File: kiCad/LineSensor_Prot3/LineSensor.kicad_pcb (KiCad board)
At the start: 2 copper layers, 113 parts, among them J1 Conn_01x04_Socket, J2 Conn_01x02_Socket, Q1 Q_Photo_NPN, Q10 Q_Photo_NPN, Q11 Q_Photo_NPN, Q12 Q_Photo_NPN, Q13 Q_Photo_NPN, Q14 Q_Photo_NPN, Q15 Q_Photo_NPN, Q16 Q_Photo_NPN, Q17 NMOS, Q2 Q_Photo_NPN, Q3 Q_Photo_NPN, Q4 Q_Photo_NPN, Q5 Q_Photo_NPN, Q6 Q_Photo_NPN, Q7 Q_Photo_NPN, Q8 Q_Photo_NPN, Q9 Q_Photo_NPN, SW2 SW_DPST_x2, U1 LM393, U2 LM393, U3 LM393, U4 LM393, U5 LM393, U6 LM393, U7 LM393, U8 LM393, U9 LM393

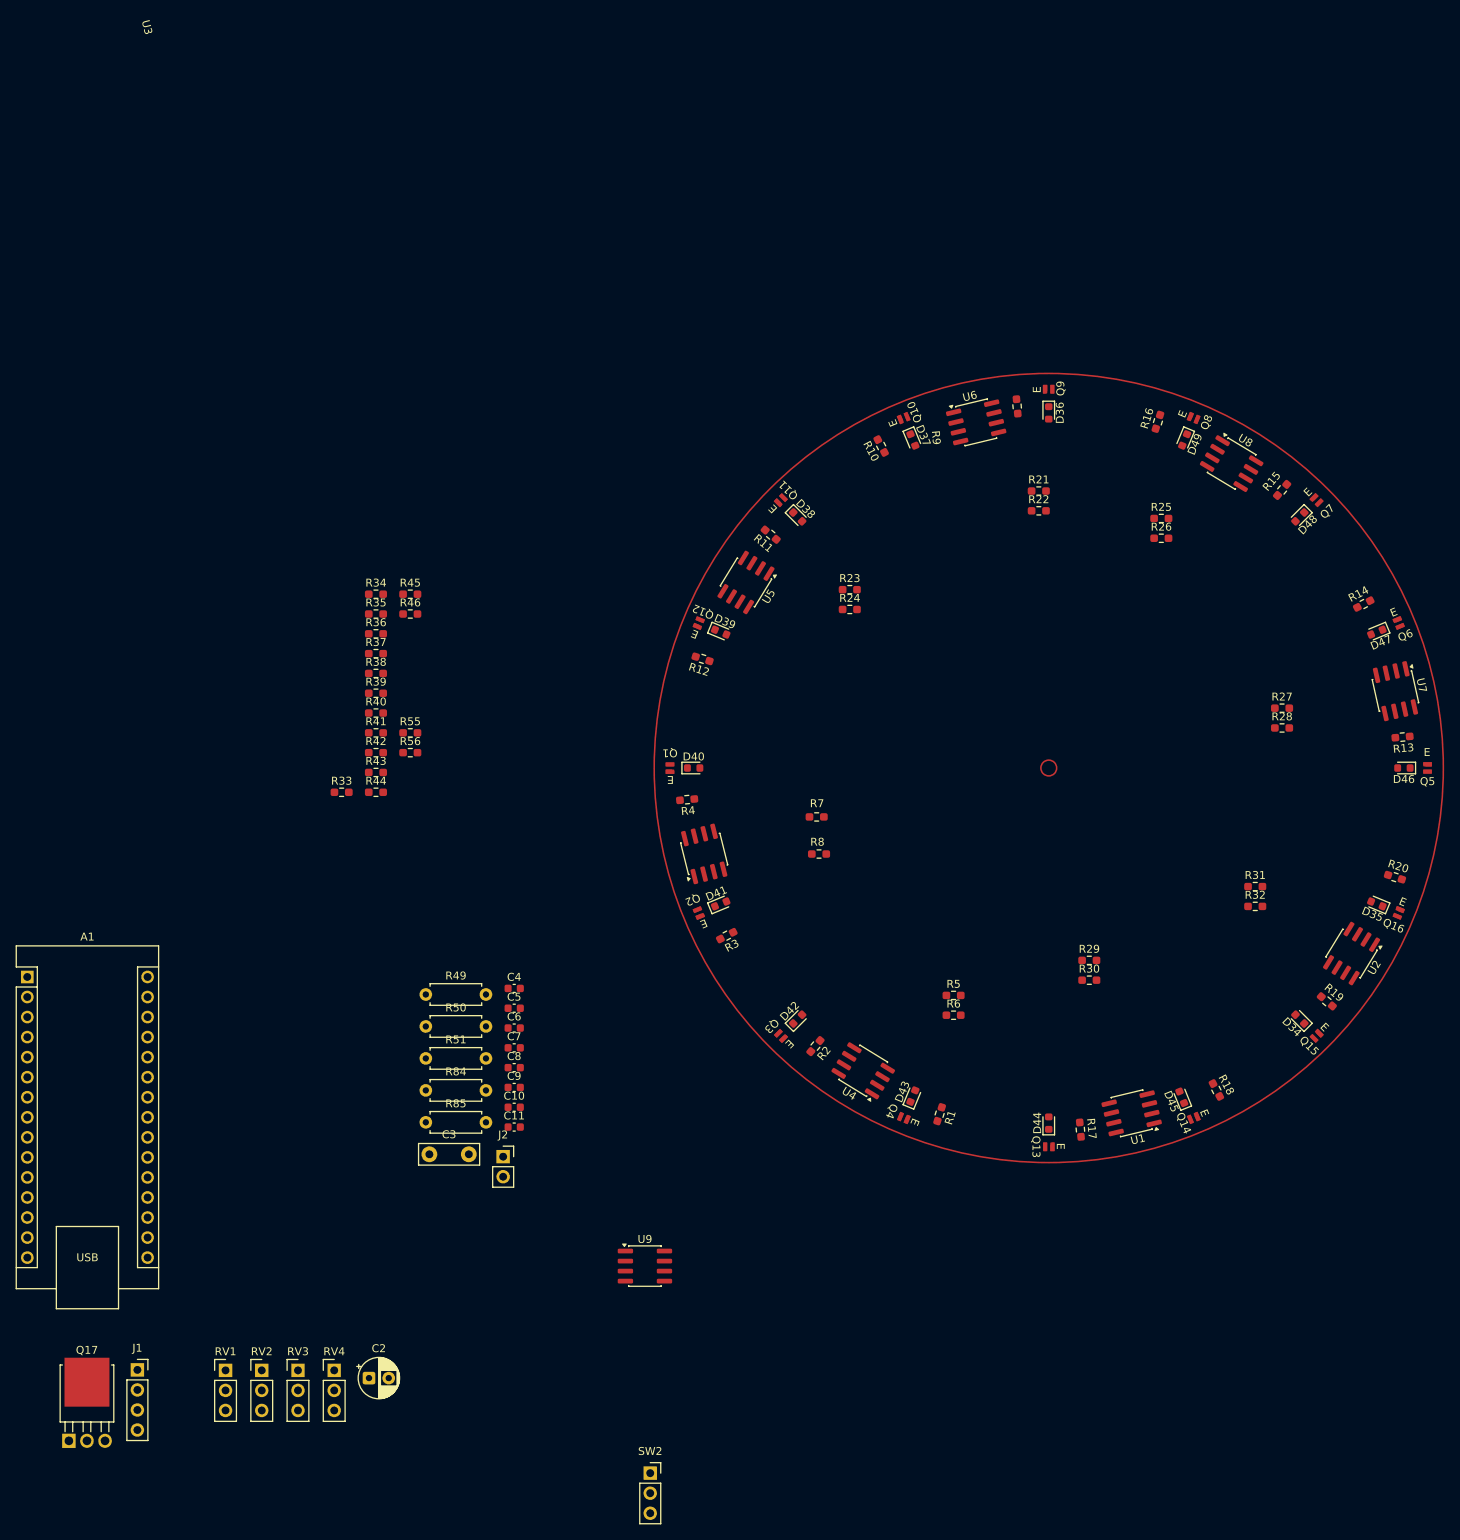
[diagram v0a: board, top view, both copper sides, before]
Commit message: 円形最低限
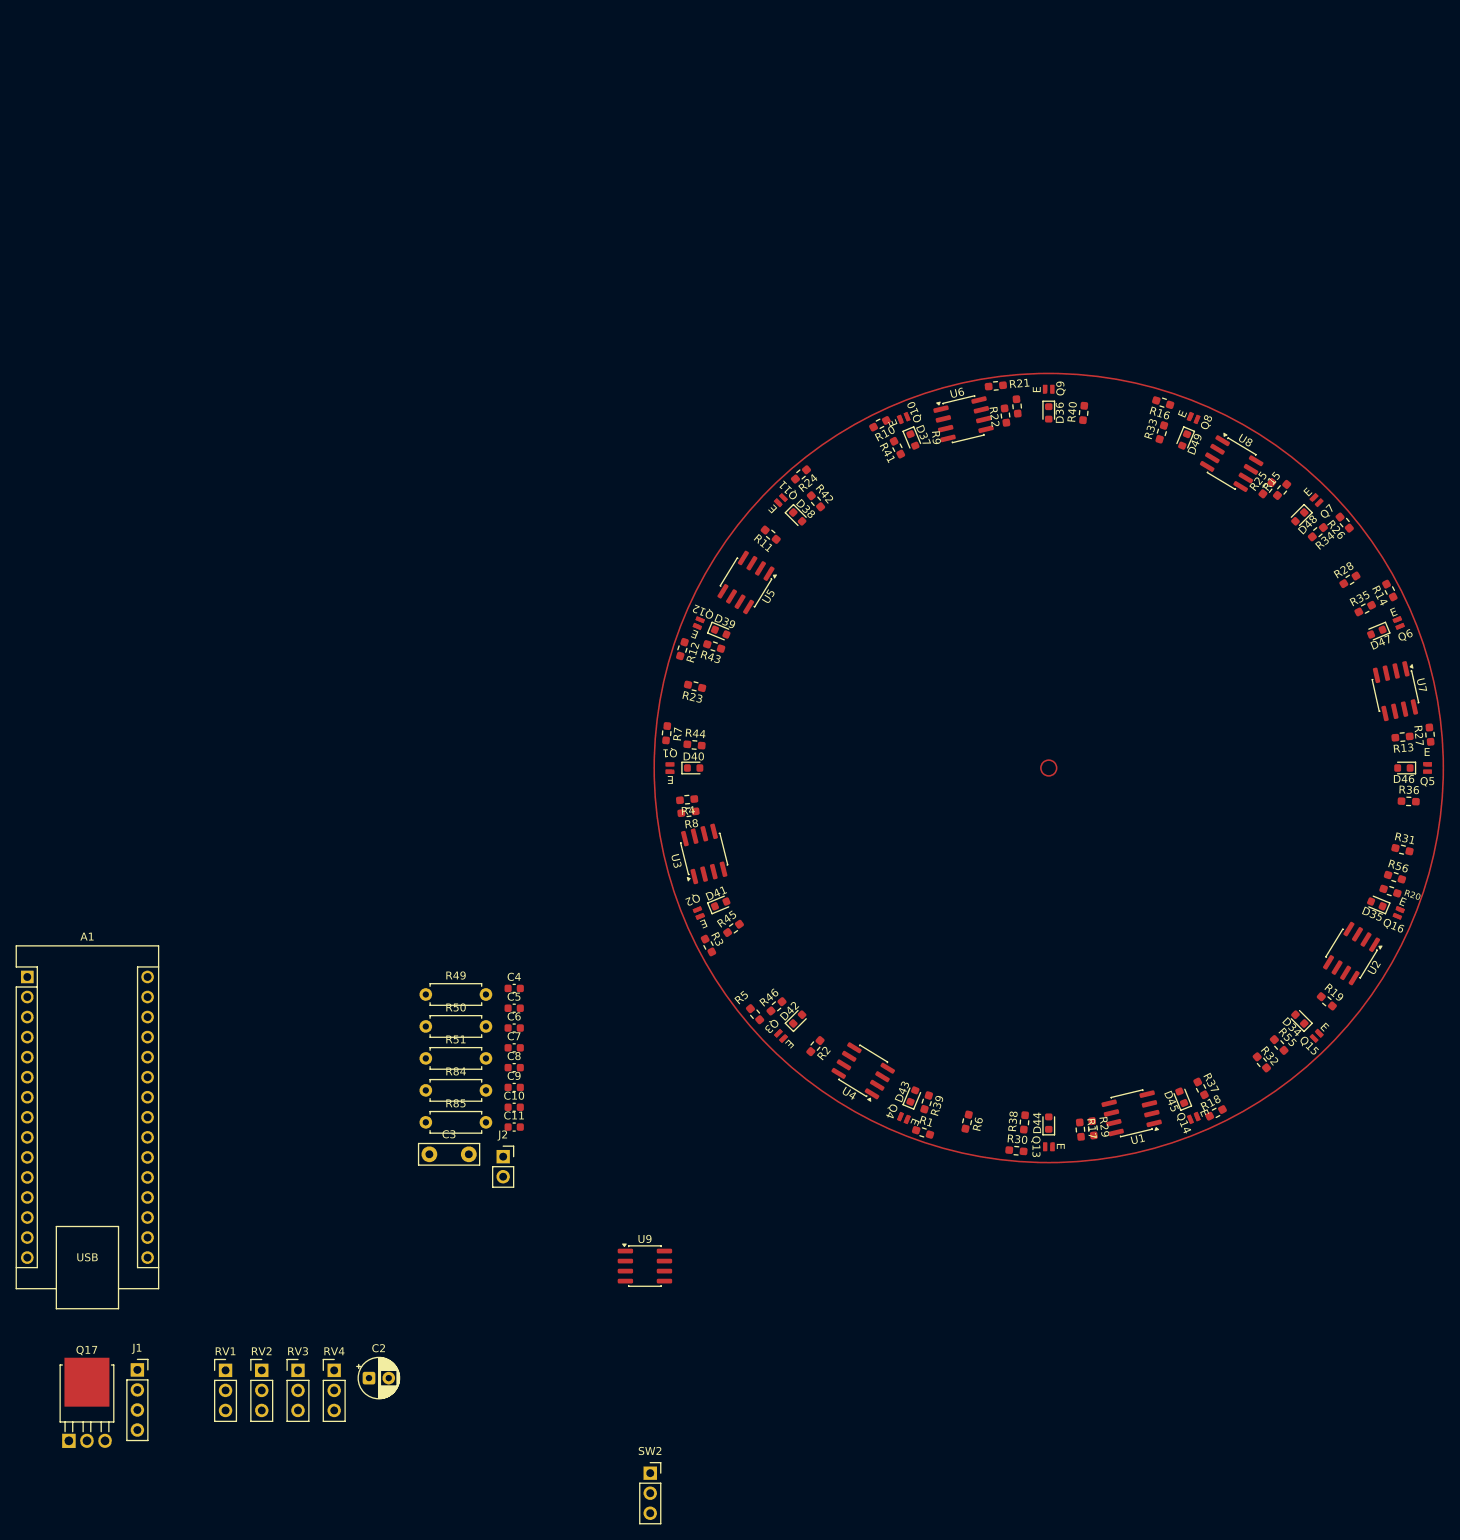
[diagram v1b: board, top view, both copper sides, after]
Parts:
- moved R36 132.6 mm to (195.6, 104.2), turned to -2 degrees
- moved R56 125.8 mm to (193.9, 113.8), turned to -17.5 degrees
- moved R35 125.4 mm to (190.1, 79.8), turned to 27.5 degrees
- moved R34 119.6 mm to (184.1, 70.1), turned to -140 degrees
- moved R37 118.2 mm to (169.3, 140.6), turned to -62.5 degrees
- moved R55 117.0 mm to (179.2, 135.1), turned to -48 degrees
- moved R33 113.5 mm to (164.3, 57.5), turned to 72.5 degrees
- moved R38 100.0 mm to (146.9, 144.9), turned to 85 degrees
- moved R40 97.4 mm to (154.4, 55.0), turned to 85 degrees
- moved R39 86.9 mm to (134.5, 142.4), turned to -107.5 degrees
- moved R41 75.3 mm to (130.8, 59.4), turned to 117.5 degrees
- moved R46 68.0 mm to (115.5, 130.2), turned to 40 degrees
- moved R42 64.2 mm to (120.5, 66.2), turned to -50 degrees
- moved R45 58.9 mm to (110.1, 120.3), turned to 35 degrees
- moved R43 45.7 mm to (107.6, 84.6), turned to 162.5 degrees
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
